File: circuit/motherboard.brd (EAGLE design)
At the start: 69.5 x 99 mm, 14 parts, among them T1 BC337

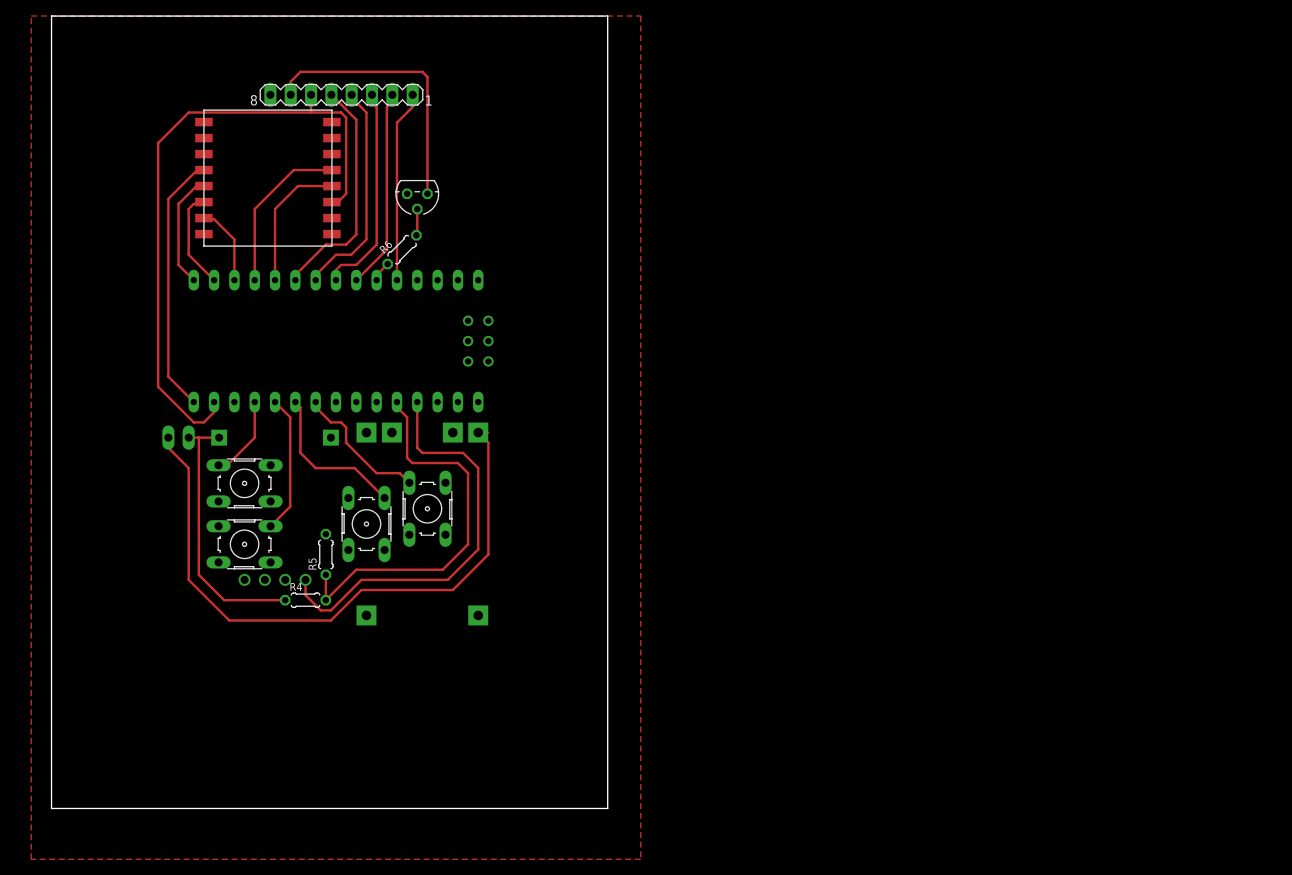
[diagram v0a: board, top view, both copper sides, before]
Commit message: Getting to be quite a serious design..
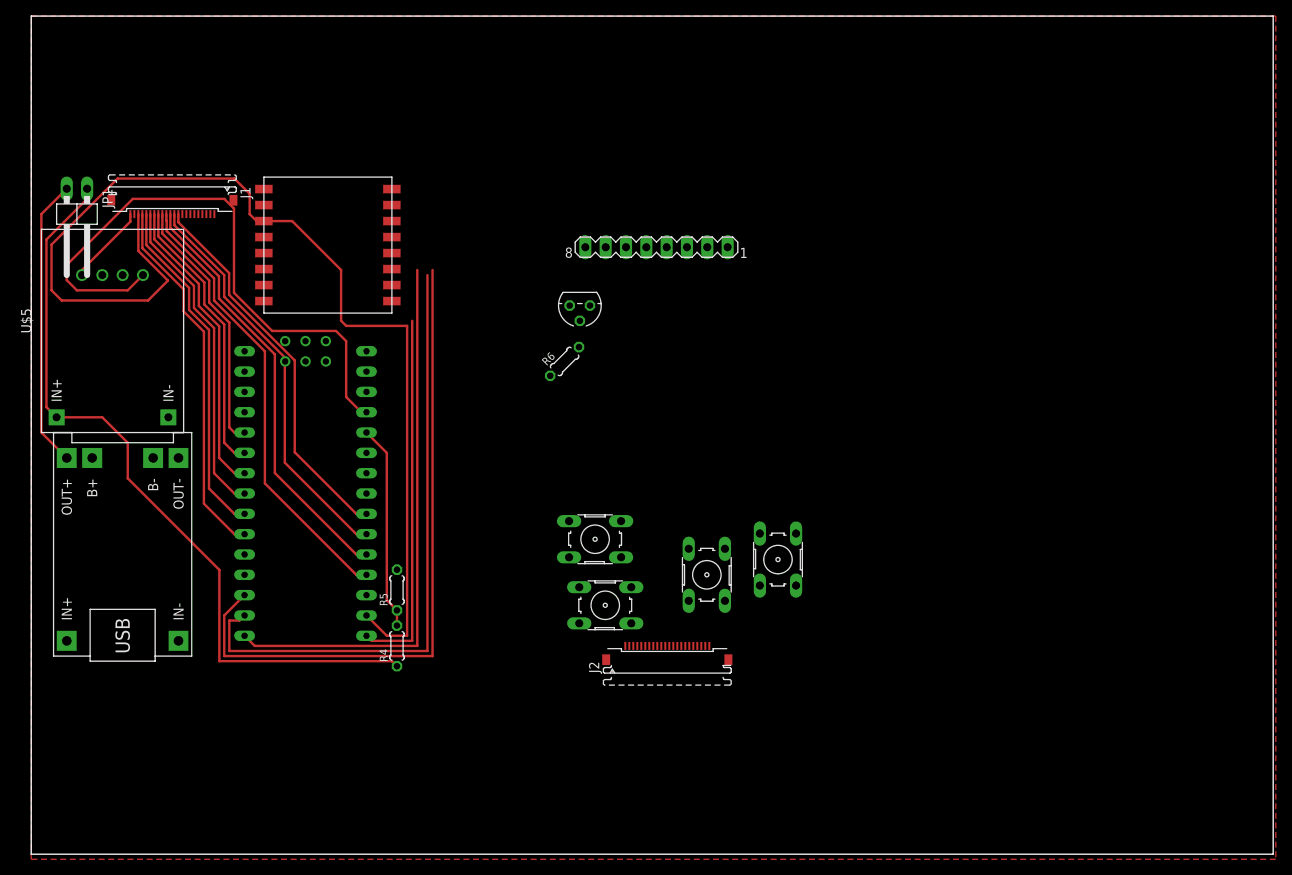
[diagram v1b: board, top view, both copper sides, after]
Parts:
- added J1, J2: XF2L-2235-1, con-omron:XF2L-2235-1
- moved S2 51.6 mm to (101.0, 17.1)
- moved S3 45.7 mm to (79.4, 11.4)
- moved S4 44.4 mm to (78.1, 19.7)
- moved DIS2 43.7 mm to (86.4, 38.1)
- moved U$3 37.6 mm to (19.1, 19.1), flipped to the top
- moved S1 35.9 mm to (92.1, 15.2)
- moved JP1 33.6 mm to (13.3, 59.7), flipped to the top
- moved U$5 31.5 mm to (17.8, 45.7), flipped to the top, turned to 90 degrees
- moved R6 24.7 mm to (74.3, 41.9)
- moved T1 24.7 mm to (76.2, 48.9)
- moved U$1 19.8 mm to (39.4, 34.3), turned to 180 degrees
- moved R4 12.8 mm to (53.3, 6.35), turned to 90 degrees
- moved U$4 11.2 mm to (44.7, 56.5), turned to 0 degrees
- moved R5 9.94 mm to (53.3, 13.3)
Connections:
- removed net N$16: JP1.2, R4.1, U$5.IN+
- new net N$17: DIS2.1, J2.9
- new net N$22: J2.12, S3.3
- new net N$25: DIS2.6, J2.3
- new net N$26: DIS2.5, J2.4
- new net N$27: DIS2.4, J2.5
- new net N$28: DIS2.3, J2.6
- new net N$29: DIS2.2, J2.7
- new net N$30: J2.13, S4.3
- new net N$32: J1.13, U$1.A0
- new net N$33: J1.12, U$1.A1
- new net N$34: J1.11, U$1.A2
- new net N$35: J1.10, U$1.A3
- net +3V3: now also J1.20; no longer DIS2.6
- net GND: now also J1.22, J2.1, S1.1, S1.2, S2.1, S2.2, S3.1, S3.2, S4.1, S4.2; no longer S1.3, S2.3, S3.3, S4.3
- net N$10: now also J1.18; no longer DIS2.4
- net N$11: now also J1.17; no longer DIS2.3
- net N$12: now also J1.16; no longer DIS2.2
- net N$13: now also J1.15; no longer R6.1
- net N$15: now also JP1.2; no longer JP1.1
- net N$18: now also JP1.1, R4.1, U$5.IN+; no longer S4.1, S4.2, U$1.A0
- net N$19: now also J2.8, R6.1; no longer S3.1, S3.2, U$1.A1
- net N$20: now also J2.10, S1.3; no longer S2.1, S2.2, U$1.A2
- net N$21: now also J2.11, S2.3; no longer S1.1, S1.2, U$1.A3
- net N$3: now also J1.19; no longer DIS2.5
- net N$9: now also J1.14; no longer DIS2.1
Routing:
- net N$18: track 10.4 -> 95.9 mm
- net N$6: track 10.0 -> 83.0 mm
- net N$5: track 12.9 -> 77.7 mm
- net +3V3: track 80.4 -> 137.2 mm
- net N$32: track 0.00 -> 56.2 mm
- net N$4: track 14.4 -> 69.1 mm
- net N$33: track 0.00 -> 53.4 mm
- net N$34: track 0.00 -> 50.7 mm
- net N$35: track 0.00 -> 47.9 mm
- net N$15: track 78.9 -> 36.3 mm
- net N$23: track 34.1 -> 0.00 mm
- net N$16: track 33.1 -> 0.00 mm
- net N$13: track 2.59 -> 35.1 mm
- net N$24: track 48.7 -> 25.7 mm
- net +5V: track 52.0 -> 74.9 mm
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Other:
- board size 69.5 x 99 mm -> 155.2 x 104.8 mm
